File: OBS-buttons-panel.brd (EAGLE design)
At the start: 144.8 x 81.2 mm, 23 parts

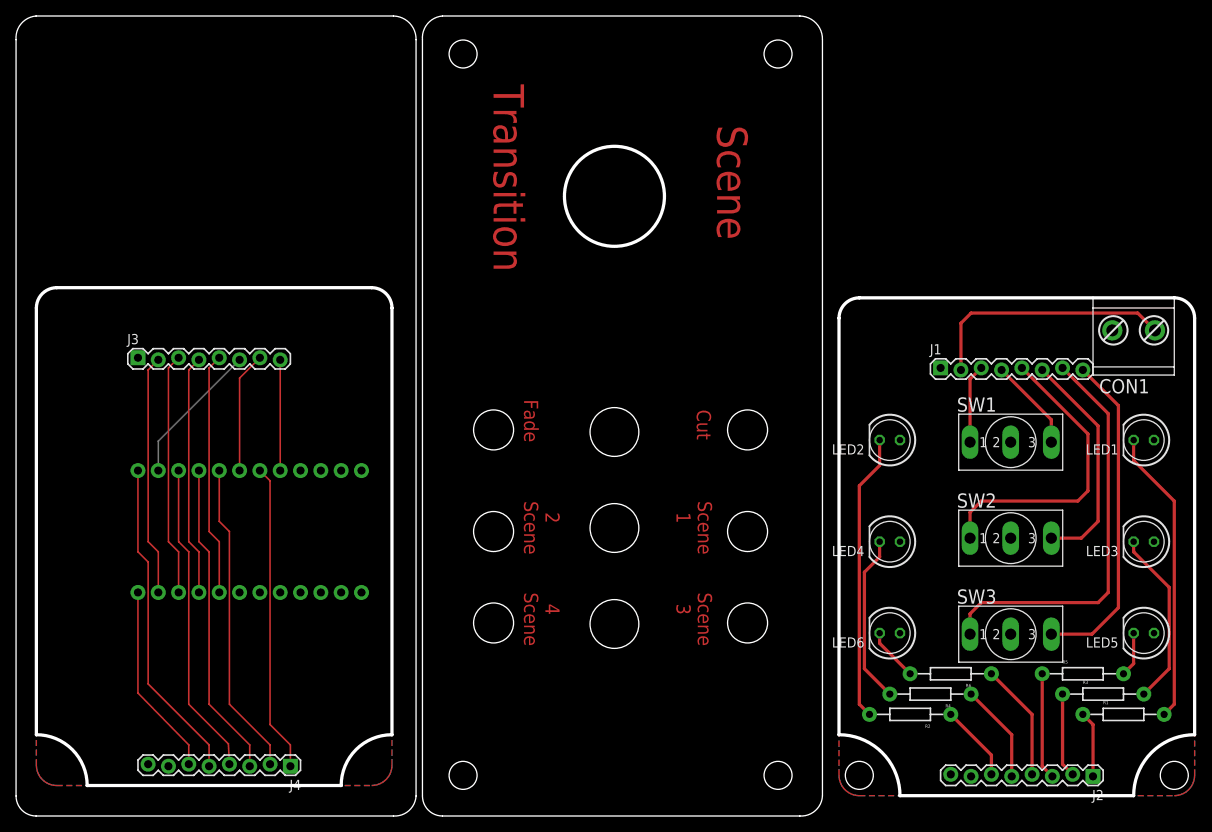
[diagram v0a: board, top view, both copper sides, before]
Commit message: initial prototype
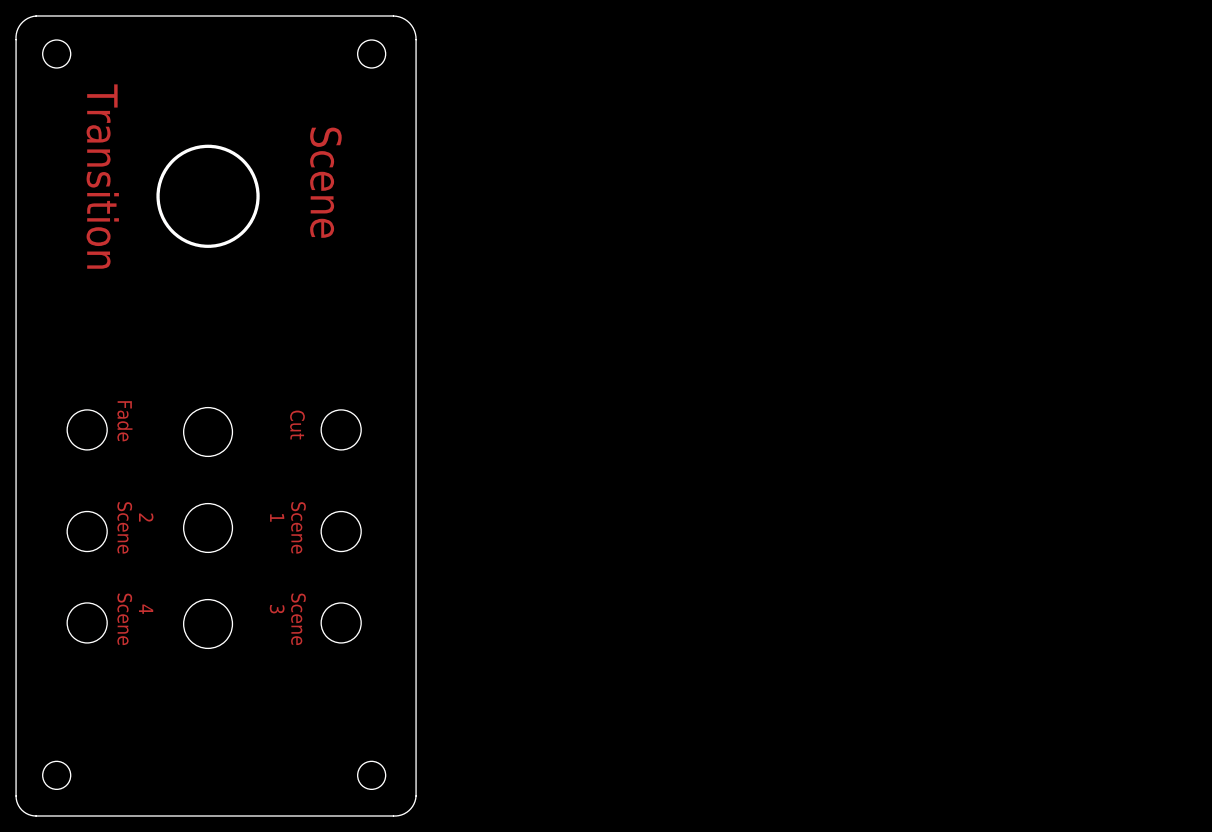
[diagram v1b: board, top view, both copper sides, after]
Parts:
- removed BOARD2: (no value), SPCoast:BOARD-SEEED10X5-NOHOLES
- removed CON1: (no value), SPCoast:MSTB2
- removed J1, J2, J3, J4: (no value), SPCoast:1X08_LOCK
- removed LED1, LED2, LED3, LED4, LED5, LED6: (no value), SPCoast:LED5MM
- removed R1, R2, R3, R4, R5, R6: (no value), SPCoast:AXIAL-0.4-RES
- removed SW1, SW2, SW3: (no value), SPCoast:SWITCH-SPDT-508
- removed U$1: ARDUINO-PRO-MICROEBAY, SPCoast:ARDUINO-PRO-MICRO
- moved BOARD1 50.8 mm to (0.00, 0.00)
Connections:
- removed net CUT: J1.3, SW1.1
- removed net CUT-LED: J2.1, R1.P$1
- removed net FADE: J1.4, SW1.3
- removed net FADE-LED: J2.6, R2.P$1
- removed net GND: CON1.1, J2.7, J2.8, J4.7, J4.8, SW1.2, SW2.2, SW3.2, U$1.GND@1, U$1.GND@2, U$1.GND@4
- removed net I1: J3.5, U$1.AD0
- removed net I2: J3.4, U$1.D13
- removed net I3: J3.3, U$1.D12
- removed net I4: J3.2, U$1.D11
- removed net I5: J3.6, U$1.D8
- removed net I6: J3.7, U$1.D4
- removed net I7: J3.8, U$1.D2
- removed net N$1: LED1.K, R1.P$2
- removed net N$2: LED2.K, R2.P$2
- removed net N$3: LED3.K, R3.P$2
- removed net N$4: LED4.K, R4.P$2
- removed net N$5: LED5.K, R5.P$2
- removed net N$6: LED6.K, R6.P$2
- removed net O1: J4.1, U$1.D3
- removed net O2: J4.2, U$1.D5
- removed net O3: J4.3, U$1.D6
- removed net O4: J4.4, U$1.D7
- removed net O5: J4.5, U$1.D9
- removed net O6: J4.6, U$1.D10
- removed net SCENE1: J1.5, SW2.1
- removed net SCENE1-LED: J2.2, R3.P$1
- removed net SCENE2: J1.6, SW2.3
- removed net SCENE2-LED: J2.5, R4.P$1
- removed net SCENE3: J1.7, SW3.1
- removed net SCENE3-LED: J2.3, R5.P$1
- removed net SCENE4: J1.8, SW3.3
- removed net SCENE4-LED: J2.4, R6.P$1
- removed net TRANSITION: CON1.2, J1.2
- removed net VCC: J1.1, J3.1, LED1.A, LED2.A, LED3.A, LED4.A, LED5.A, LED6.A, U$1.5V
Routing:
- net SCENE3: track 51.4 -> 0.00 mm
- net SCENE4: track 41.3 -> 0.00 mm
- net O5: track 40.6 -> 0.00 mm
- net O3: track 39.6 -> 0.00 mm
- net O2: track 39.3 -> 0.00 mm
- net O4: track 39.3 -> 0.00 mm
- net O1: track 38.5 -> 0.00 mm
- net SCENE1: track 37.9 -> 0.00 mm
- net N$1: track 36.9 -> 0.00 mm
- net N$2: track 35.9 -> 0.00 mm
- net TRANSITION: track 31.5 -> 0.00 mm
- net I3: track 30.4 -> 0.00 mm
- net I1: track 30.4 -> 0.00 mm
- net I4: track 30.1 -> 0.00 mm
- net I2: track 30.1 -> 0.00 mm
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- removed copper zone on layer 16, net GND
- removed copper zone on layer 1, net VCC
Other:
- board size 144.8 x 81.2 mm -> 50 x 100 mm
